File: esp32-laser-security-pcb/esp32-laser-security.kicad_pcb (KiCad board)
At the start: 2 copper layers, 46.5 x 52 mm, 13 parts, among them J1 Conn_01x06, SW1 SW_Push

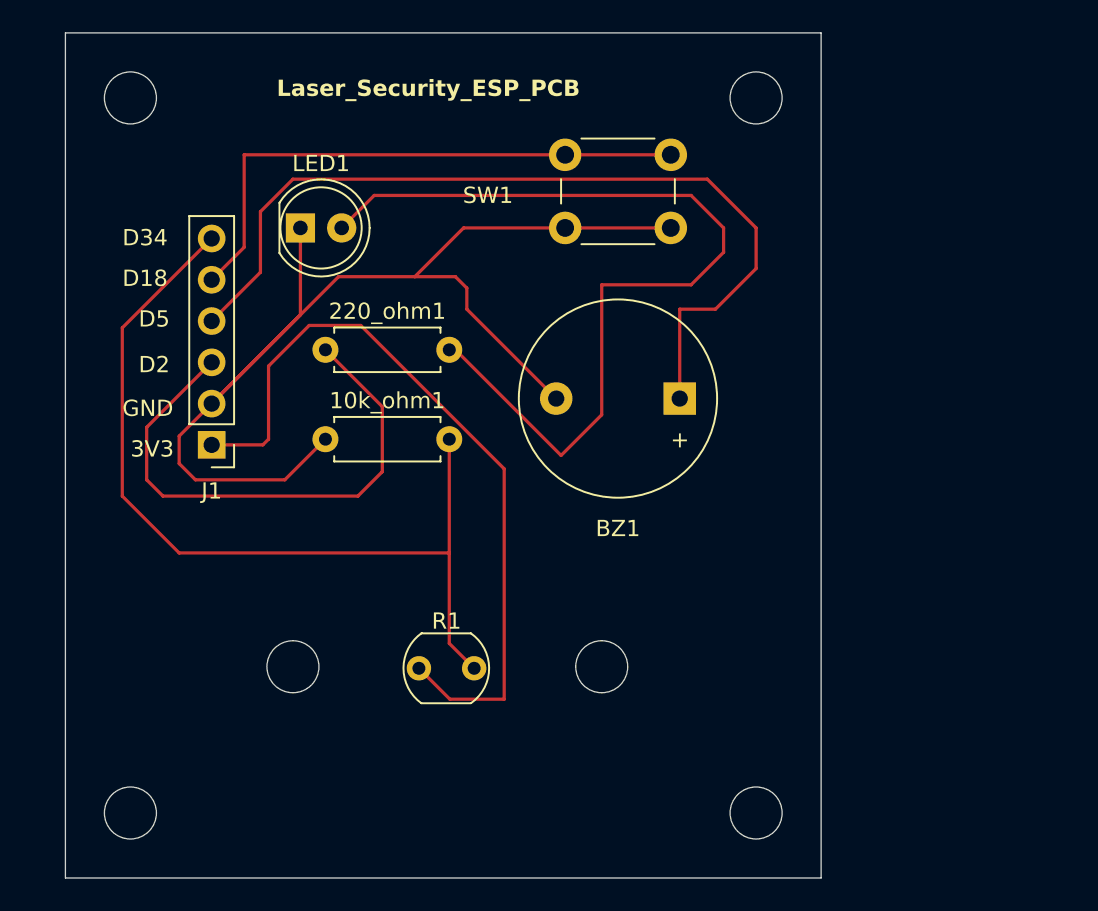
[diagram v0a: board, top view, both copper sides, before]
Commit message: updated pcb
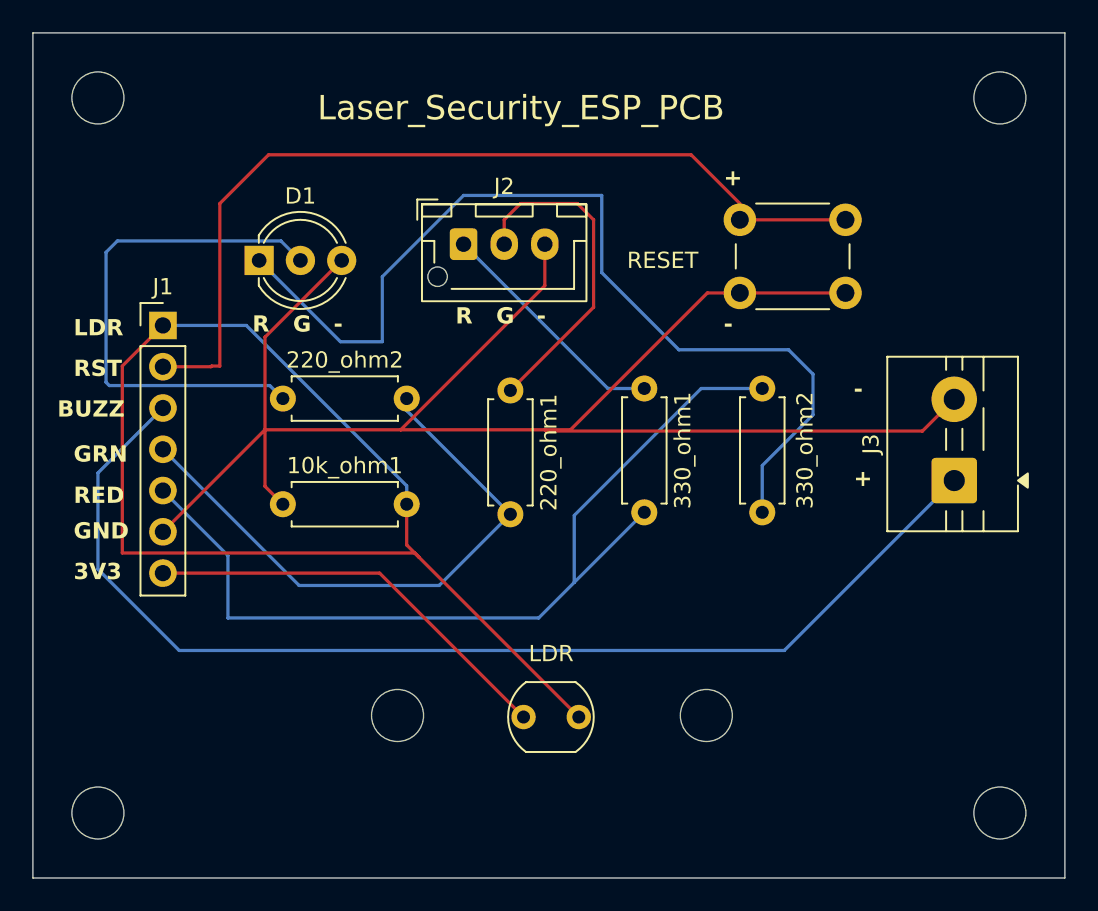
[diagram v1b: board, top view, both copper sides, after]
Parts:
- removed BZ1: Buzzer, Buzzer_Beeper:Buzzer_12x9.5RM7.6
- removed LED1: LED, LED_THT:LED_D5.0mm
- added 220_ohm2: R, Resistor_THT:R_Axial_DIN0207_L6.3mm_D2.5mm_P7.62mm_Horizontal, F.Cu at (97.4, 83.5)
- added 330_ohm1: R, Resistor_THT:R_Axial_DIN0207_L6.3mm_D2.5mm_P7.62mm_Horizontal, F.Cu at (119.6, 82.9)
- added 330_ohm2: R, Resistor_THT:R_Axial_DIN0207_L6.3mm_D2.5mm_P7.62mm_Horizontal, F.Cu at (126.9, 90.5)
- added D1: LED_Dual_AAK, LED_THT:LED_D5.0mm-3, F.Cu at (95.9, 75.0)
- added J2: LED_connector, Connector_JST:JST_XH_B3B-XH-AM_1x03_P2.50mm_Vertical, F.Cu at (108.5, 74.0)
- added J3: Conn_01x02_Pin, TerminalBlock:TerminalBlock_MaiXu_MX126-5.0-02P_1x02_P5.00mm, F.Cu at (138.7, 88.5)
- J1: value Conn_01x06 -> Conn_01x07; footprint Connector_PinHeader_2.54mm:PinHeader_1x06_P2.54mm_Vertical -> Connector_PinHeader_2.54mm:PinHeader_1x07_P2.54mm_Vertical
- moved REF** 15.0 mm to (141.5, 109.0)
- moved REF** 15.0 mm to (141.5, 65.0)
- moved 220_ohm1 11.7 mm to (111.4, 83.0), turned to -90 degrees
- moved RESET 11.5 mm to (125.5, 72.5)
- moved J1 7.94 mm to (90.0, 79.0), turned to 0 degrees
- moved LDR 7.10 mm to (112.2, 103.1)
- moved REF** 7.10 mm to (123.4, 103.0)
- moved REF** 7.10 mm to (104.4, 103.0)
- moved 10k_ohm1 4.78 mm to (97.4, 90.0)
- moved REF** 2.00 mm to (86.0, 65.0)
- moved REF** 2.00 mm to (86.0, 109.0)
- renumbered R1 to LDR, SW1 to RESET
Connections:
- 10k_ohm1 pad 1: Net-(BZ1--) -> /GND
- 10k_ohm1 pad 2: Net-(J1-Pin_6) -> /D34
- 220_ohm1 pad 1: Net-(J1-Pin_3) -> Net-(J2-Pin_2)
- 220_ohm1 pad 2: Net-(LED1-A) -> /D4
- J1 pad 1: Net-(J1-Pin_1) -> /D34
- J1 pad 2: Net-(BZ1--) -> /D18
- J1 pad 3: Net-(J1-Pin_3) -> /D5
- J1 pad 4: Net-(BZ1-+) -> /D4
- J1 pad 5: Net-(J1-Pin_5) -> /D2
- J1 pad 6: Net-(J1-Pin_6) -> /GND
- LDR pad 1: Net-(J1-Pin_1) -> /3V3
- LDR pad 2: Net-(J1-Pin_6) -> /D34
- RESET pad 1: Net-(J1-Pin_5) -> /D18
- RESET pad 2: Net-(BZ1--) -> /GND
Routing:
- net /GND: track 0.00 -> 106.6 mm
- net Net-(BZ1--): track 73.3 -> 0.00 mm
- net /D34: track 0.00 -> 71.1 mm
- net /D5: track 0.00 -> 70.7 mm
- net Net-(D1-A1): track 0.00 -> 59.4 mm
- net /D2: track 0.00 -> 56.7 mm
- net Net-(LED1-A): track 56.1 -> 0.00 mm
- net /D18: track 0.00 -> 55.5 mm
- net Net-(J1-Pin_6): track 54.4 -> 0.00 mm
- net Net-(BZ1-+): track 54.3 -> 0.00 mm
- net Net-(J1-Pin_1): track 47.5 -> 0.00 mm
- net /D4: track 0.00 -> 36.4 mm
- net Net-(J1-Pin_5): track 34.8 -> 0.00 mm
- net Net-(J1-Pin_3): track 33.4 -> 0.00 mm
- net Net-(D1-A2): track 0.00 -> 32.0 mm
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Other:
- board size 46.5 x 52 mm -> 63.5 x 52 mm
- board text added: "+"
- board text added: "-"
- board text added: "BUZZ"
- board text added: "G"
- board text added: "GRN"
- board text added: "LDR"
- board text added: "R"
- board text added: "RED"
- board text added: "RST"
- board text removed: "D18"
- board text removed: "D2"
- board text removed: "D34"
- board text removed: "D5"
